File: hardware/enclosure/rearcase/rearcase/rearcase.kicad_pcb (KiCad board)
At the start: 2 copper layers, 42.5 x 23 mm, 1 part

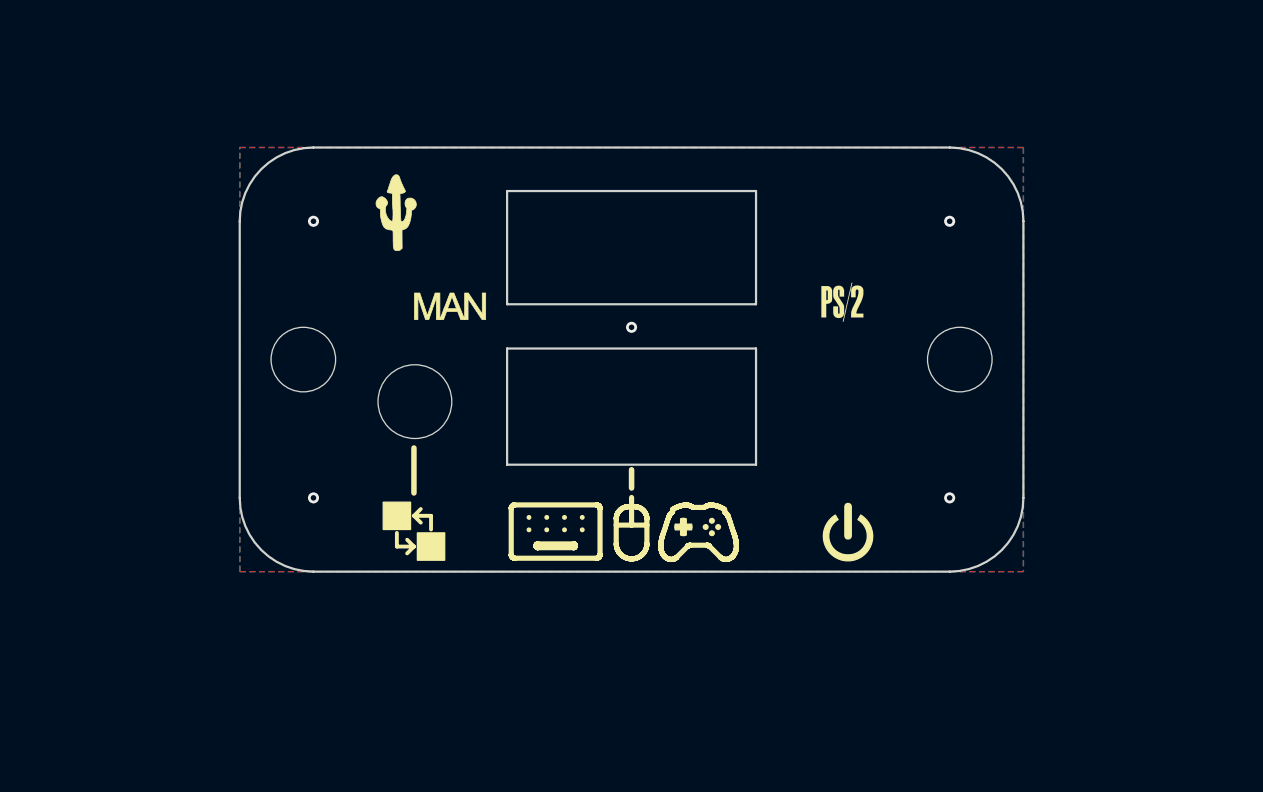
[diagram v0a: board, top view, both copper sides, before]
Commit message: serial enclosure
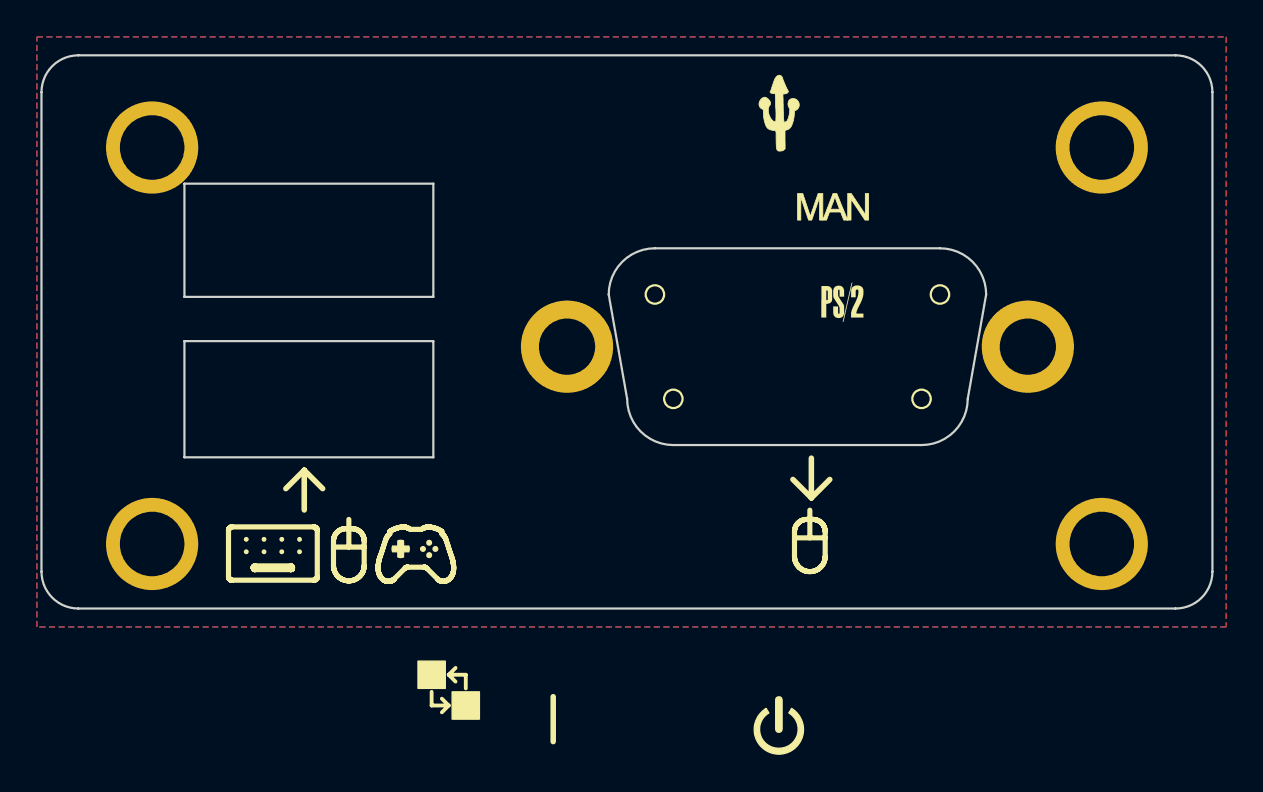
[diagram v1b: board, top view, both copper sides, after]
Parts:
- removed the REF** at (154.0, 98.0)
- added REF**: rearpanell, ps2pcb:rearpanell, F.Cu at (153.8, 96.5)
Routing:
- net GND: vias 5 -> 0
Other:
- board size 42.5 x 23 mm -> 63.5 x 30 mm
